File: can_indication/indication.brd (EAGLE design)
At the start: 160 x 100 mm, 51 parts, among them CON1 SM04B-GHS-TB, CON2 SM04B-GHS-TB, U1 STM32F103CB

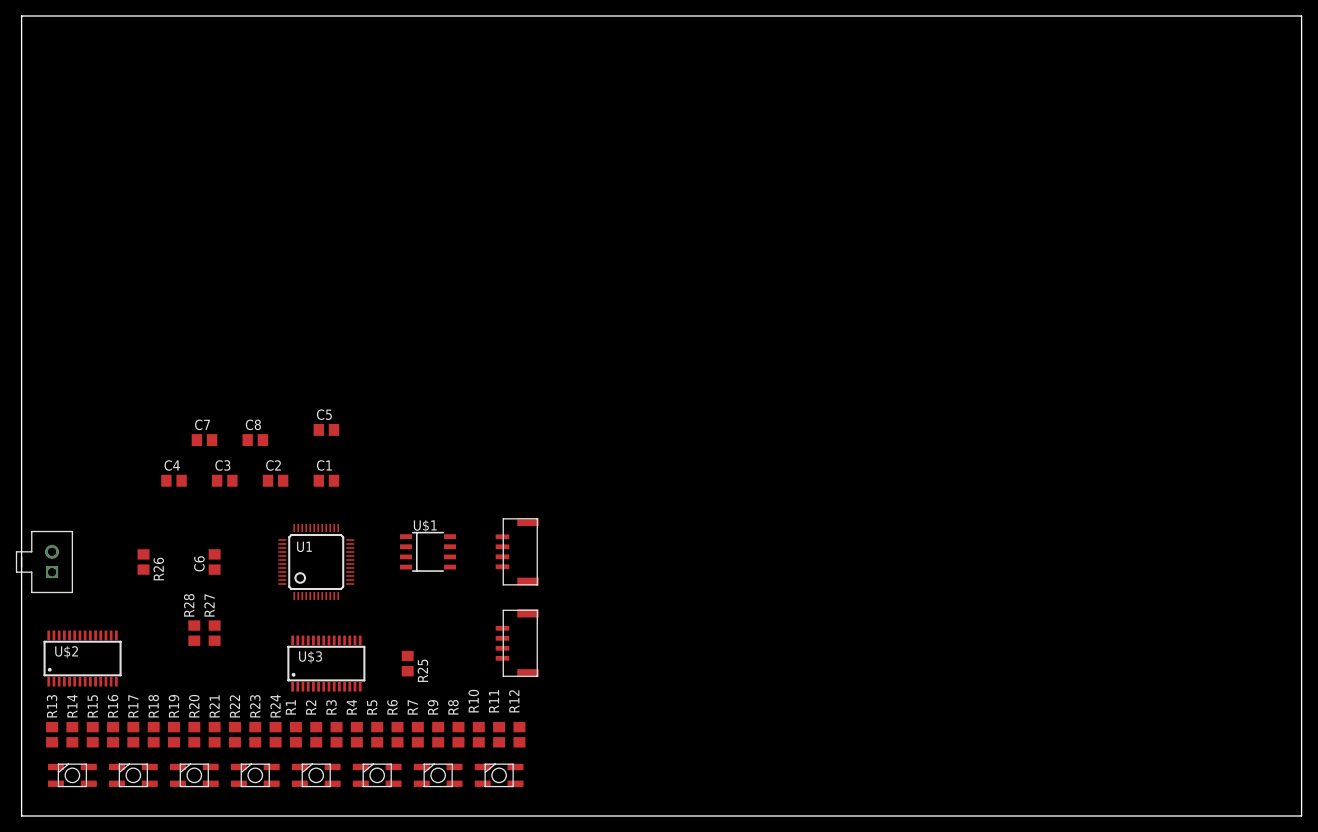
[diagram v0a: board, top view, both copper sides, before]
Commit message: Finished placement.
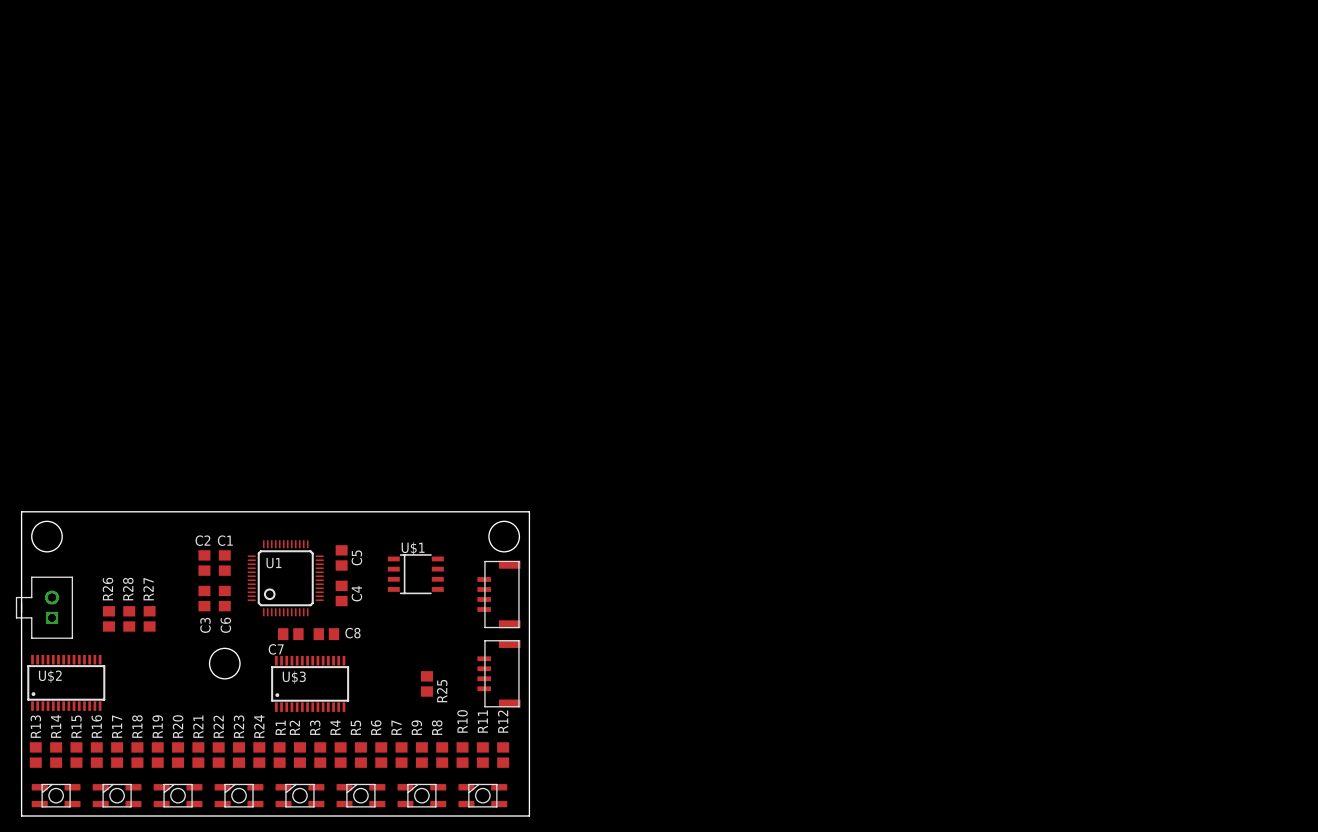
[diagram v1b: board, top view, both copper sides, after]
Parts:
- moved C7 26.6 mm to (33.7, 22.7), turned to 180 degrees
- moved C8 25.8 mm to (38.1, 22.7)
- moved C4 25.3 mm to (40.0, 27.8), turned to 270 degrees
- moved C1 16.3 mm to (25.4, 31.6), turned to 90 degrees
- moved C5 16.1 mm to (40.0, 32.3), turned to 90 degrees
- moved C3 14.9 mm to (22.9, 27.2), turned to 270 degrees
- moved C2 13.6 mm to (22.9, 31.6), turned to 90 degrees
- moved R27 8.32 mm to (16.0, 24.6)
- moved R28 8.32 mm to (13.5, 24.6)
- moved R26 8.32 mm to (10.9, 24.6), turned to 90 degrees
- moved CON2 5.80 mm to (58.7, 27.7)
- moved U$4 5.71 mm to (3.81, 26.0)
- moved C6 4.75 mm to (25.4, 27.2), turned to 270 degrees
- moved CON1 4.44 mm to (58.7, 17.8)
- moved U1 4.32 mm to (33.0, 29.7)
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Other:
- board size 160 x 100 mm -> 63.5 x 38 mm
